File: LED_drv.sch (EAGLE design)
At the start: 54 parts, among them IC1 LM3409, IC2 LM393D, Q2 IRF840, T1 IRLR9343PBF, T2 BC847, T4 BT169, T5 BT169, T6 TLP266J

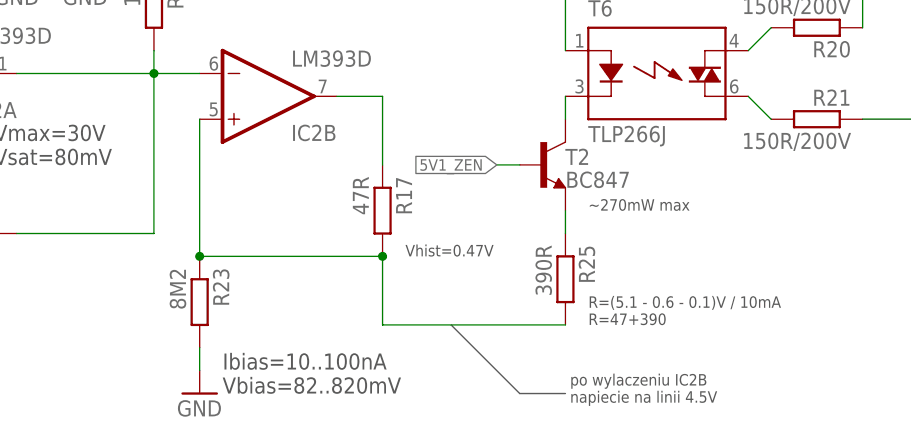
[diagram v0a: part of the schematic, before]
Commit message: Additional corrections
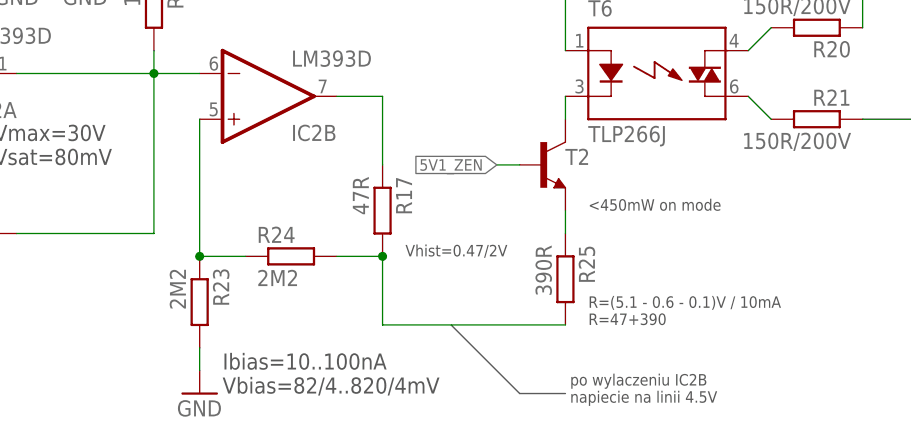
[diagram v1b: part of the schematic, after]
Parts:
- added R24: 2M2, resistor:R-EU_R0805
- R23: value 8M2 -> 2M2
- T2: value BC847 -> (none); device transistor:BC847 -> transistor:BCX56-NPN-SOT89-BCE
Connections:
- new net N$21: IC2B.+IN, R23.1, R24.1
- net N$30: now also R24.2; no longer IC2B.+IN, R23.1
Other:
- note added: "<450mW on mode"
- note added: "Ibias=10..100nA Vbias=82/4..820/4mV"
- note added: "Vhist=0.47/2V"
- note removed: "Ibias=10..100nA Vbias=82..820mV"
- note removed: "Vhist=0.47V"
- note removed: "~270mW max"
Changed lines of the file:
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@@
 <part name="SUPPLY1" library="supply2" deviceset="V+" device="" value="10-42V"/>
 <part name="GND14" library="supply1" deviceset="GND" device=""/>
-<part name="R23" library="resistor" deviceset="R-EU_" device="R0805" value="8M2"/>
-<part name="T2" library="transistor" deviceset="BC847" device=""/>
+<part name="R23" library="resistor" deviceset="R-EU_" device="R0805" value="2M2"/>
+<part name="T2" library="transistor" deviceset="*-NPN-" device="SOT89-BCE" technology="BCX56"/>
 <part name="R25" library="resistor" deviceset="R-EU_" device="R0805" value="390R"/>
 <part name="SUPPLY3" library="supply2" deviceset="V+" device="" value="10-42V"/>
@@
 <part name="GND15" library="supply1" deviceset="GND" device=""/>
 <part name="C9" library="rcl" deviceset="CPOL-US" device="E3.5-8" value="100uF/50V"/>
+<part name="R24" library="resistor" deviceset="R-EU_" device="R0805" value="2M2"/>
 </parts>
 <sheets>
@@
 Vsat=80mV</text>
 <text x="279.4" y="-45.72" size="1.778" layer="97">Ibias=10..100nA
-Vbias=82..820mV</text>
+Vbias=82/4..820/4mV</text>
 <text x="320.04" y="-38.1" size="1.27" layer="97">R=(5.1 - 0.6 - 0.1)V / 10mA
 R=47+390</text>
-<text x="320.04" y="-25.4" size="1.27" layer="97">~270mW max</text>
-<text x="299.72" y="-30.48" size="1.27" layer="97">Vhist=0.47V</text>
+<text x="320.04" y="-25.4" size="1.27" layer="97">&lt;450mW on mode</text>
+<text x="299.72" y="-30.48" size="1.27" layer="97">Vhist=0.47/2V</text>
 <text x="318.008" y="-46.736" size="1.27" layer="97">po wylaczeniu IC2B
 napiecie na linii 4.5V</text>
@@
 <instance part="GND15" gate="1" x="289.56" y="12.7"/>
 <instance part="C9" gate="G$1" x="289.56" y="25.4"/>
+<instance part="R24" gate="G$1" x="287.02" y="-30.48"/>
 </instances>
 <busses>
@@
 <net name="N$30" class="0">
 <segment>
-<pinref part="IC2" gate="B" pin="+IN"/>
-<pinref part="R23" gate="G$1" pin="1"/>
-<wire x1="276.86" y1="-30.48" x2="276.86" y2="-15.24" width="0.1524" layer="91"/>
 <pinref part="R25" gate="G$1" pin="2"/>
 <wire x1="317.5" y1="-38.1" x2="297.18" y2="-38.1" width="0.1524" layer="91"/>
 <pinref part="R17" gate="G$1" pin="2"/>
 <wire x1="297.18" y1="-30.48" x2="297.18" y2="-38.1" width="0.1524" layer="91"/>
-<wire x1="276.86" y1="-30.48" x2="297.18" y2="-30.48" width="0.1524" layer="91"/>
-<junction x="276.86" y="-30.48"/>
 <junction x="297.18" y="-30.48"/>
+<pinref part="R24" gate="G$1" pin="2"/>
+<wire x1="292.1" y1="-30.48" x2="297.18" y2="-30.48" width="0.1524" layer="91"/>
 </segment>
 </net>
@@
 </segment>
 </net>
+<net name="N$21" class="0">
+<segment>
+<pinref part="IC2" gate="B" pin="+IN"/>
+<pinref part="R24" gate="G$1" pin="1"/>
+<pinref part="R23" gate="G$1" pin="1"/>
+<wire x1="276.86" y1="-30.48" x2="281.94" y2="-30.48" width="0.1524" layer="91"/>
+<junction x="276.86" y="-30.48"/>
+<wire x1="276.86" y1="-30.48" x2="276.86" y2="-15.24" width="0.1524" layer="91"/>
+</segment>
+</net>

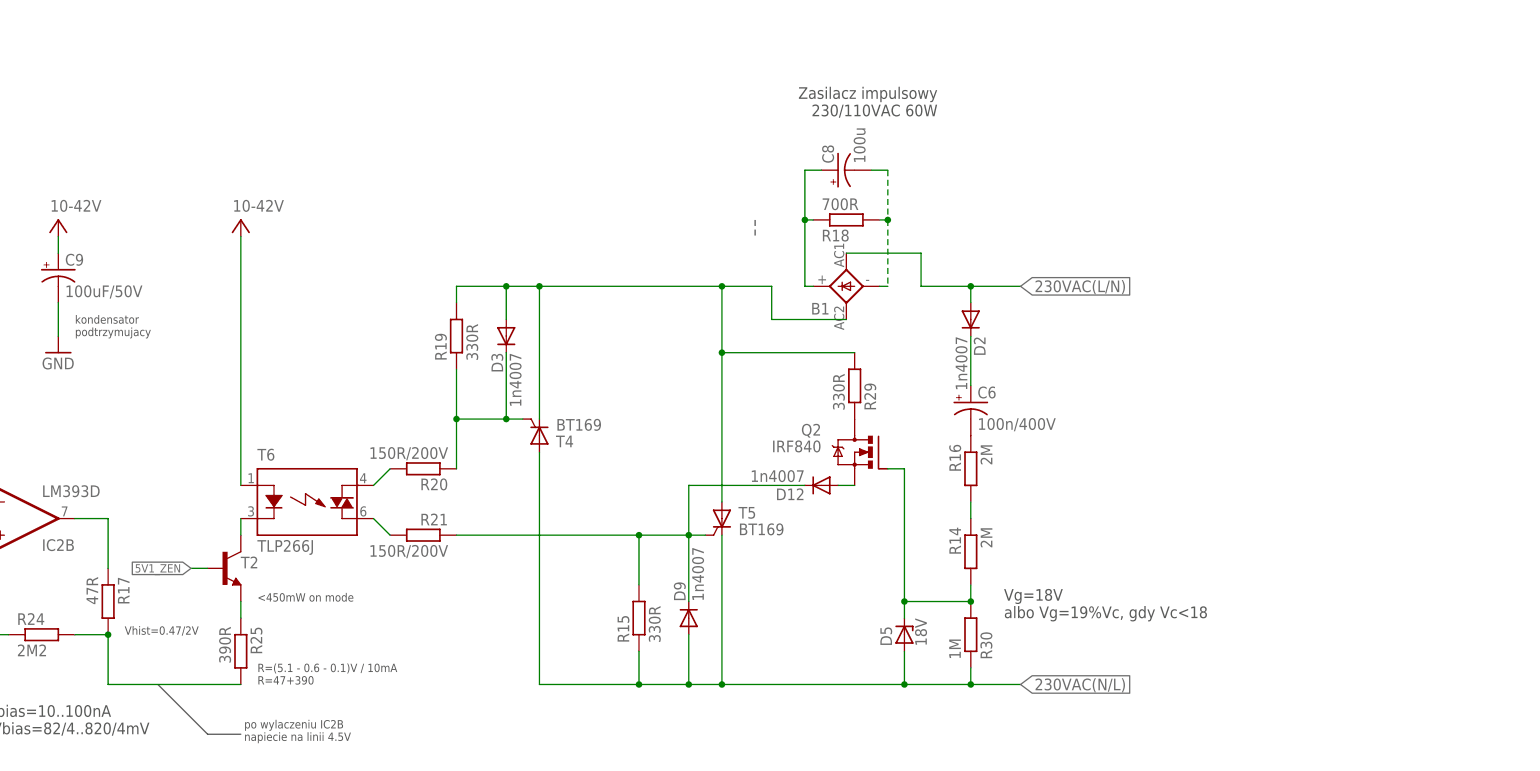
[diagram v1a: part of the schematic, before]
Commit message: Mains side PCB layout
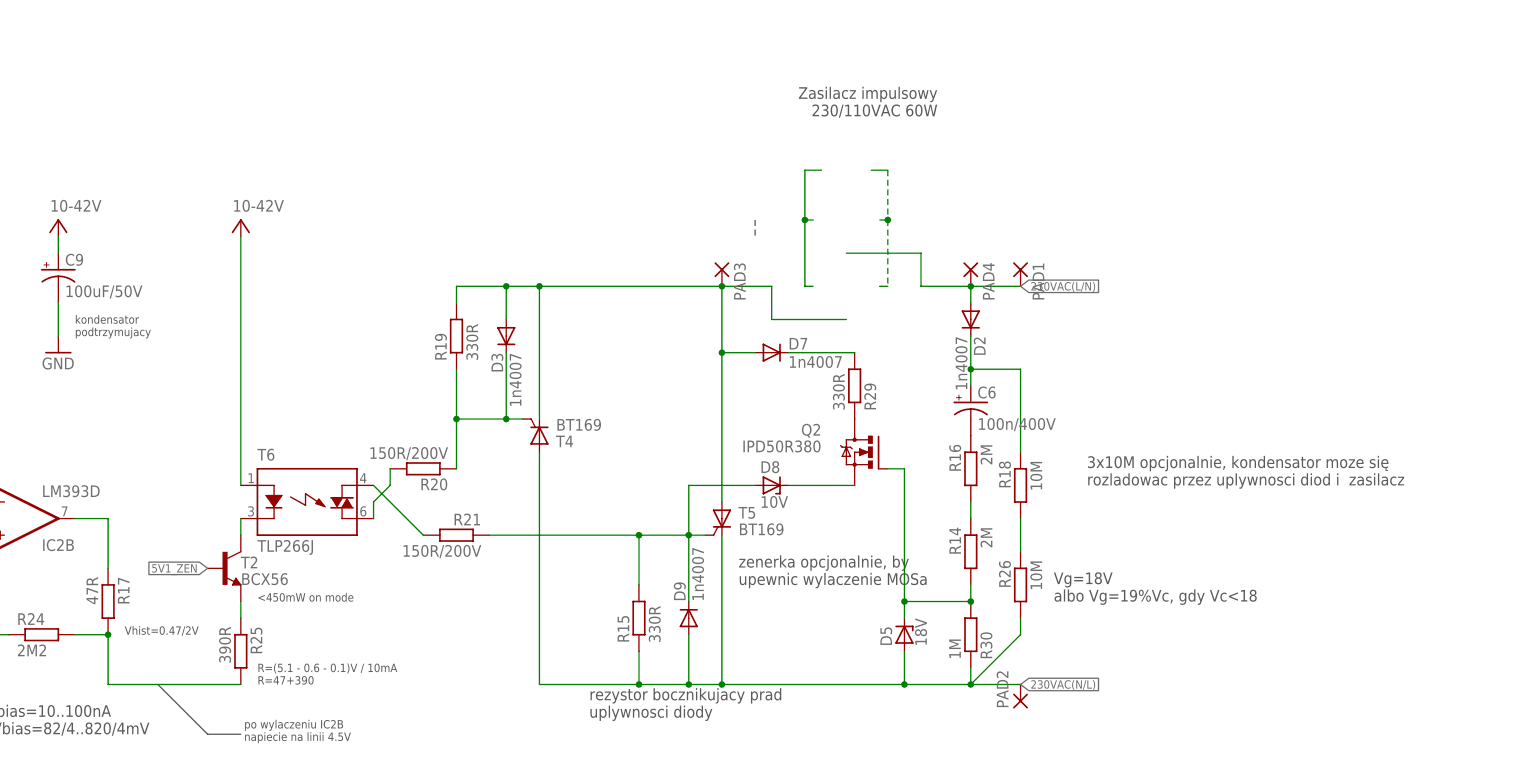
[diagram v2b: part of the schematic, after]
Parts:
- removed B1: (no value), rectifier:FBP1,5
- removed C8: 100u, rcl:CPOL-USE3.5-8
- removed D12: 1n4007, diode:DIODE-DO-214AC
- added D7: 1n4007, diode:DIODE-DO-214AC
- added D8: 10V, diode:ZENER-DIODESOD80C
- added PAD1, PAD2, PAD3, PAD4: (no value), wirepad:SMD5
- added R26: 10M, rcl:R-EU_R1206
- Q2: value IRF840 -> IPD50R380; device transistor-fet:IRF840 -> miscrel:IPD50R380
- R18: value 700R -> 10M
- T2: value (none) -> BCX56; device transistor:BCX56-NPN-SOT89-BCE -> miscrel:BCX56
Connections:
- removed net N$17: B1.+, C8.+, R18.1
- removed net N$18: B1.-, C8.-, R18.2
- new net N$24: D7.C, R29.2
- new net N$33: D8.C, Q2.S
- net 230VAC(L/N): now also PAD1.P, PAD4.P; no longer B1.AC2
- net 230VAC(N/L): now also PAD2.P, R26.2
- net N$14: now also R18.1
- net N$16: now also R21.2, T6.DS1; no longer D12.C, D9.C, R15.2, R21.1, T5.G
- net N$25: now also R20.2; no longer R21.2
- net N$26: now also R18.2, R26.1; no longer R20.2, T6.DS1
- net N$39: now also D8.A, D9.C, R15.2, R21.1, T5.G; no longer D12.A, Q2.S
- net NAH: now also D7.A, PAD3.P; no longer B1.AC1, R29.2
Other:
- note added: "3x10M opcjonalnie, kondensator moze się rozladowac przez uplywnosci diod i zasilacz"
- note added: "rezystor bocznikujacy prad uplywnosci diody"
- note added: "zenerka opcjonalnie, by upewnic wylaczenie MOSa"
- moved on the sheet: Q2, R18, R21
